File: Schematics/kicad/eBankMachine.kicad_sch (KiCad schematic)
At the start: 14 parts, among them J1 Limit Switch, J2 Conn_01x04_Pin, J3 Conn_01x04_Pin, J4 Keypad, J6 IR sensor drop, J7 IR emitter receive, J8 IR sensor receive, J9 IR emitter drop, M1 Motor_Servo, U1 ESP32-S3-MINI-1

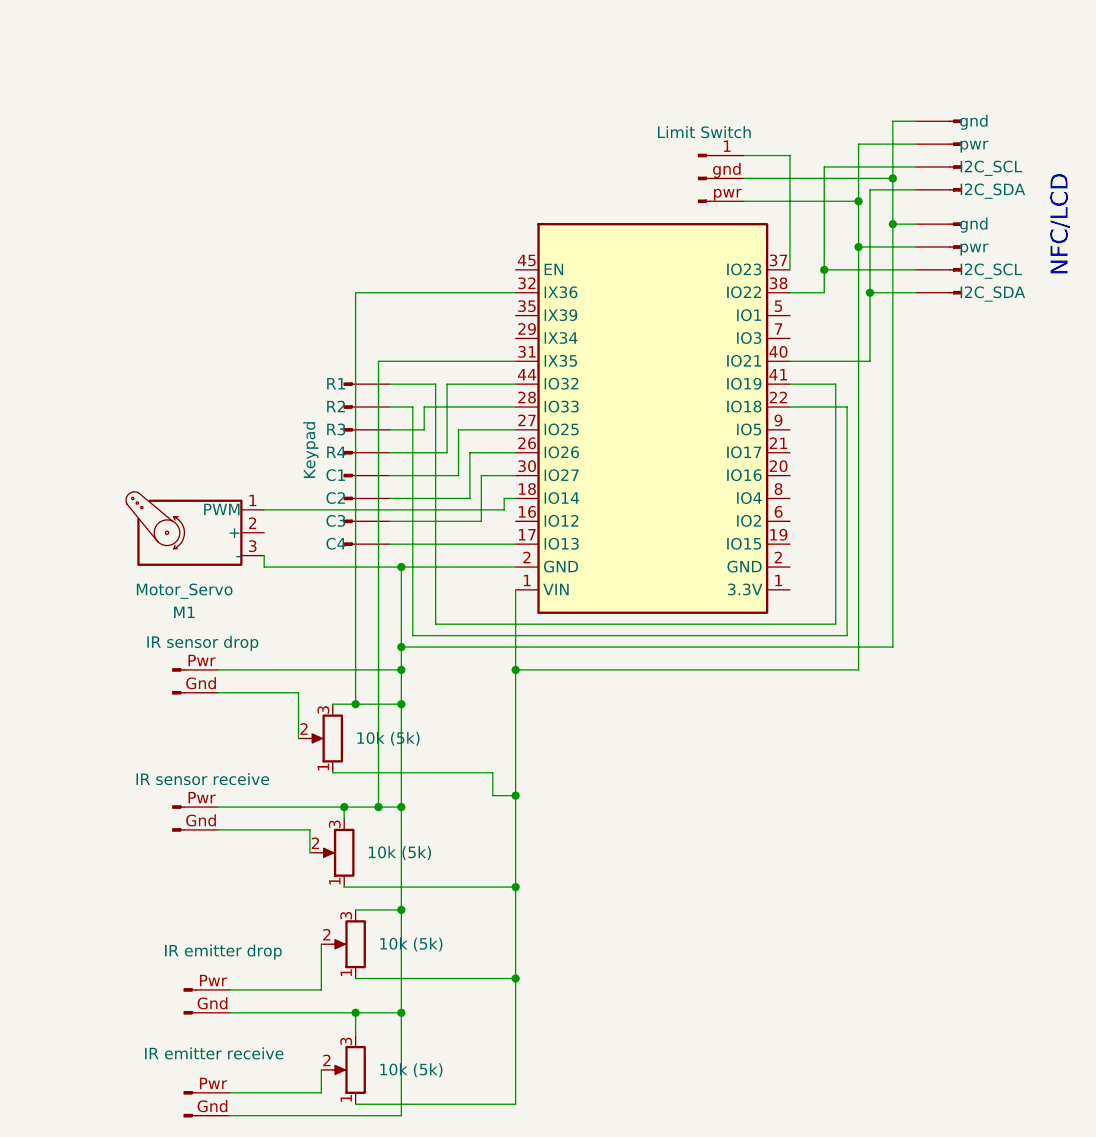
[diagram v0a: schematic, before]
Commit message: schematic updates
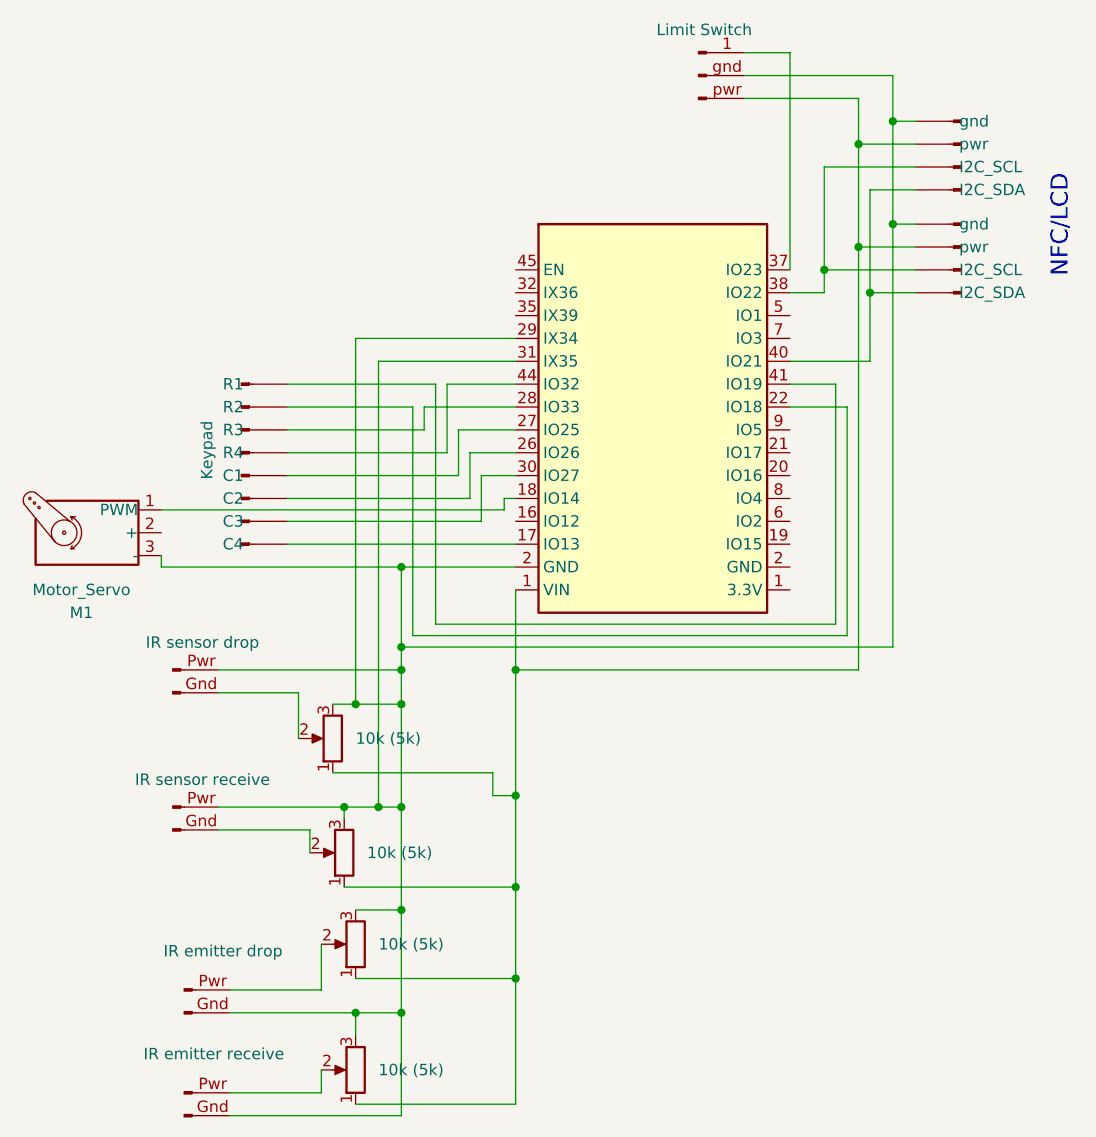
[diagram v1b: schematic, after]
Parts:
- J1, M1: footprint (none) -> Connector_PinHeader_2.54mm:PinHeader_1x03_P2.54mm_Vertical
- J2, J3: footprint (none) -> Connector_PinHeader_2.54mm:PinHeader_1x04_P2.54mm_Vertical
- J4: footprint (none) -> Connector_PinHeader_2.54mm:PinHeader_1x08_P2.54mm_Vertical
- J6, J7, J8, J9: footprint (none) -> Connector_PinHeader_2.54mm:PinHeader_1x02_P2.54mm_Vertical
- RV1, RV5, RV6, RV7: footprint (none) -> Resistor_THT:R_Axial_DIN0204_L3.6mm_D1.6mm_P2.54mm_Vertical
- U1: footprint RF_Module:ESP32-S2-MINI-1 -> RF_Module:ESP32-C3-DevKitM-1
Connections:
- net at U1.1 (3.3V): now also J1.pwr (Pin_3), J2.3 (pwr), J3.3 (pwr), RV1.1, RV5.1, RV6.1, RV7.1
- net at U1.2 (GND): now also U1.42 (GND), U1.43 (GND), U1.46 (GND), U1.47 (GND), U1.48 (GND), U1.49 (GND), U1.50 (GND), U1.51 (GND), U1.52 (GND), U1.53 (GND), U1.54 (GND), U1.55 (GND), U1.56 (GND), U1.57 (GND), U1.58 (GND), U1.59 (GND), U1.60 (GND), U1.61 (GND), U1.62 (GND), U1.63 (GND), U1.64 (GND), U1.65 (GND)
- net at J1.gnd (Pin_2), J2.4 (gnd), J3.4 (gnd)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: now also U1.29 (IX34); no longer U1.32 (IX36)
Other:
- moved on the sheet: M1
